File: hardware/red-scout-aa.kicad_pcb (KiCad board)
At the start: 2 copper layers, 61 x 70.5 mm, 31 parts, among them P1 SNAP, P2 SNAP, P3 SNAP, P4 SNAP, P5 SNAP, P6 SNAP, P7 SNAP, P8 SNAP, U1 SM200

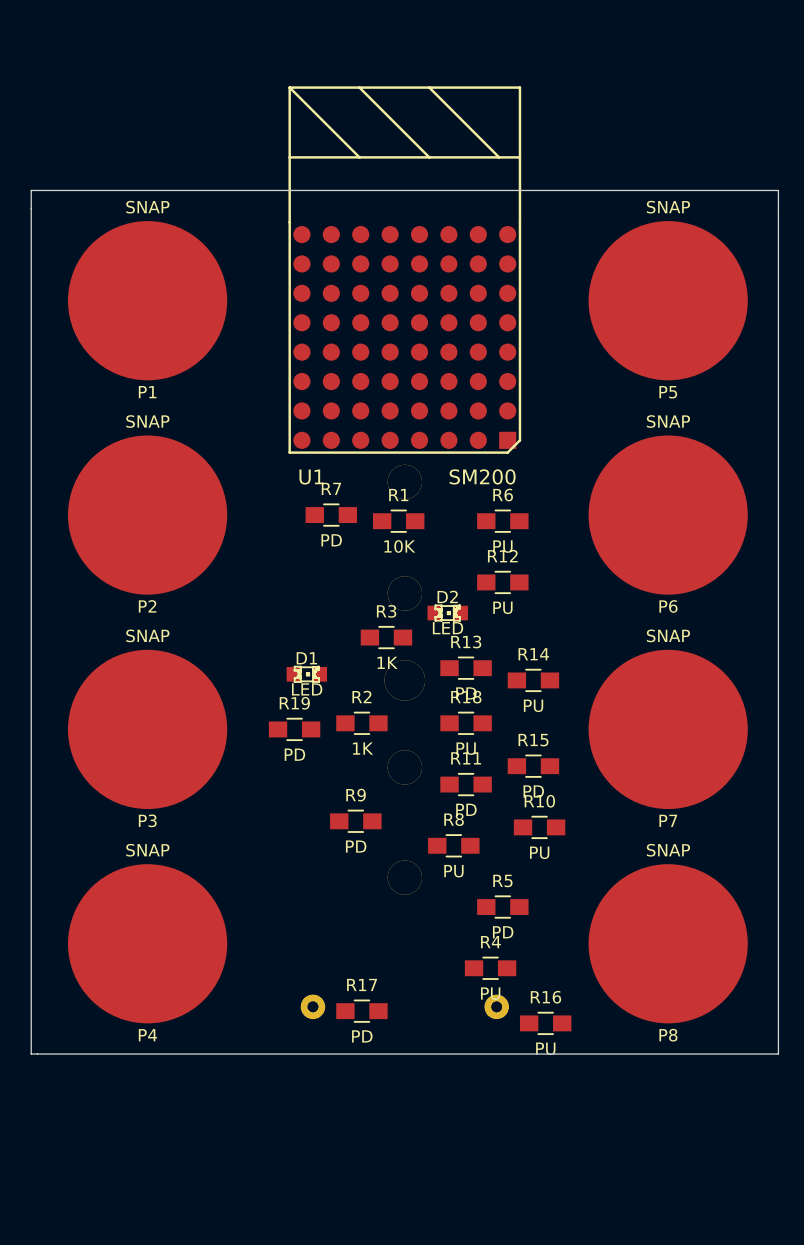
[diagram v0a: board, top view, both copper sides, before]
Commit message: Finished placing and routing board.
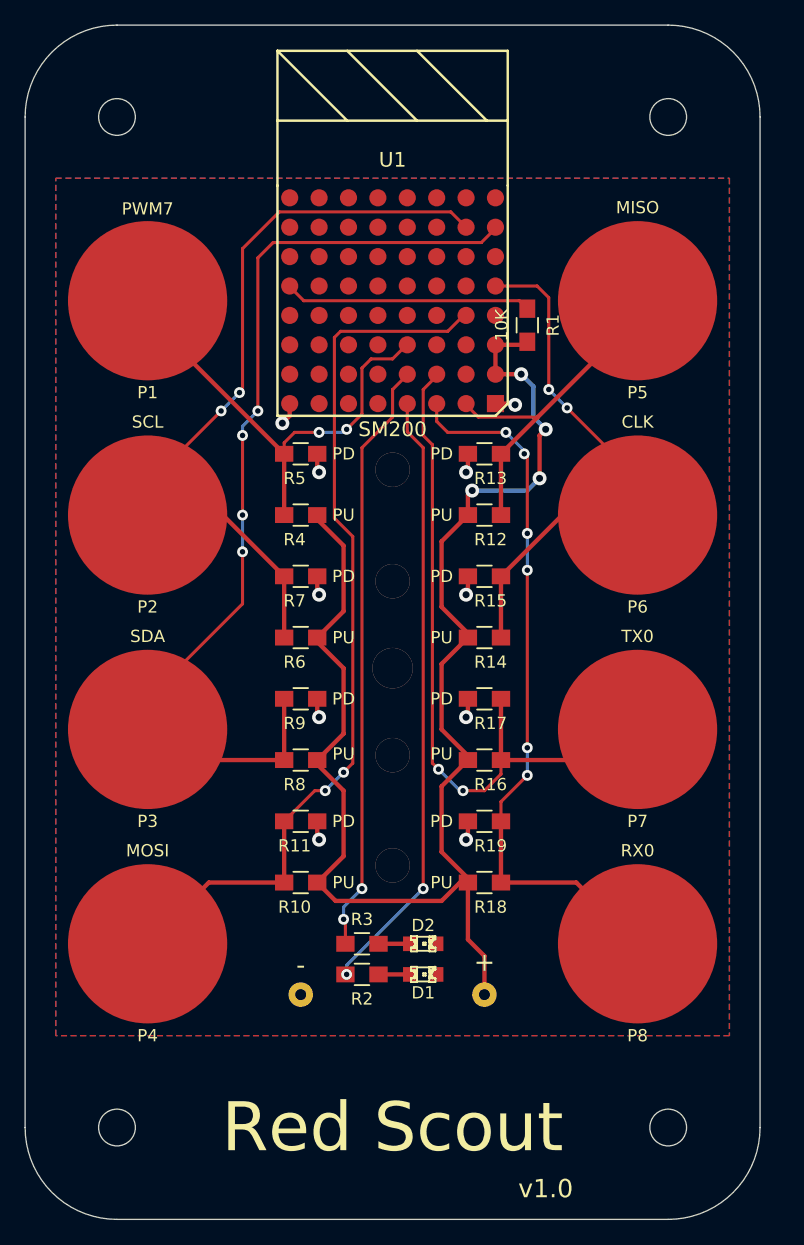
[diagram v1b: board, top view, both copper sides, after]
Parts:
- added MountingHole_3mm: VAL**, Mounting_Holes:MountingHole_3mm, F.Cu at (147.5, 45.0)
- added MountingHole_3mm: VAL**, Mounting_Holes:MountingHole_3mm, F.Cu at (102.5, 45.0)
- added MountingHole_3mm: VAL**, Mounting_Holes:MountingHole_3mm, F.Cu at (102.5, 127.5)
- added MountingHole_3mm: VAL**, Mounting_Holes:MountingHole_3mm, F.Cu at (147.5, 127.5)
- P1: value SNAP -> PWM7
- P2: value SNAP -> SCL
- P3: value SNAP -> SDA
- P4: value SNAP -> MOSI
- P5: value SNAP -> MISO
- P6: value SNAP -> CLK
- P7: value SNAP -> TX0
- P8: value SNAP -> RX0
- moved R5 40.5 mm to (117.5, 72.5)
- moved R4 40.1 mm to (117.5, 77.5)
- moved R17 27.4 mm to (132.5, 92.5), turned to 180 degrees
- moved D2 27.1 mm to (127.5, 112.5)
- moved D1 26.3 mm to (127.5, 115.0)
- moved R3 25.1 mm to (122.5, 112.5)
- moved R16 22.1 mm to (132.5, 97.5), turned to 180 degrees
- moved R2 20.5 mm to (122.5, 115.0)
- moved R10 20.0 mm to (117.5, 107.5)
- moved R1 19.1 mm to (136.0, 62.0), turned to 270 degrees
- moved R6 19.0 mm to (117.5, 87.5)
- moved R13 17.6 mm to (132.5, 72.5), turned to 180 degrees
- moved R19 17.2 mm to (132.5, 102.5), turned to 180 degrees
- moved R15 16.0 mm to (132.5, 82.5), turned to 180 degrees
- moved R8 14.3 mm to (117.5, 97.5)
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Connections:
- U1 pad D3: PWM6 -> PWM7
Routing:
- net VCC: track 0.00 -> 118.7 mm, vias 0 -> 4
- net SDA: track 0.00 -> 79.9 mm, vias 0 -> 4
- net MOSI: track 0.00 -> 72.7 mm, vias 0 -> 2
- net SCL: track 0.00 -> 63.2 mm, vias 0 -> 2
- net RX0: track 0.00 -> 59.1 mm, vias 0 -> 6
- net TX0: track 0.00 -> 57.9 mm, vias 0 -> 2
- net PWM5: track 0.00 -> 49.8 mm, vias 0 -> 2
- net PWM6: track 0.00 -> 48.7 mm, vias 0 -> 2
- net SPICLK: track 0.00 -> 43.7 mm, vias 0 -> 2
- net PWM7: track 0.00 -> 38.6 mm, vias 0 -> 2
- net MISO: track 0.00 -> 28.5 mm
- net Net-(R1-Pad1): track 0.00 -> 20.2 mm
- net GND: track 0.00 -> 16.0 mm, vias 0 -> 10
- net Net-(D2-Pad1): track 0.00 -> 2.60 mm
- net Net-(D1-Pad1): track 0.00 -> 2.60 mm
- added copper zone on B.Cu, net GND
- added copper zone on F.Cu, net GND
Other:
- board size 61 x 70.5 mm -> 60 x 97.5 mm
- net class BGA added: clearance 0.254, trace_width 0.254, via_dia 0.889, via_drill 0.635
- net class Power added: clearance 0.254, trace_width 0.356, via_dia 1.14, via_drill 0.889
- board text added: "+"
- board text added: "-"
- board text added: "Red Scout"
- board text added: "v1.0"
